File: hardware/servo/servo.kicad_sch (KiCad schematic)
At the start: 51 parts, among them J2 Conn_ARM_SWD_TagConnect_TC203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, U3 DRV8876PWPR, U4 STM32G030F6P6, U5 SIT3088EEUA, U6 SRV05-4

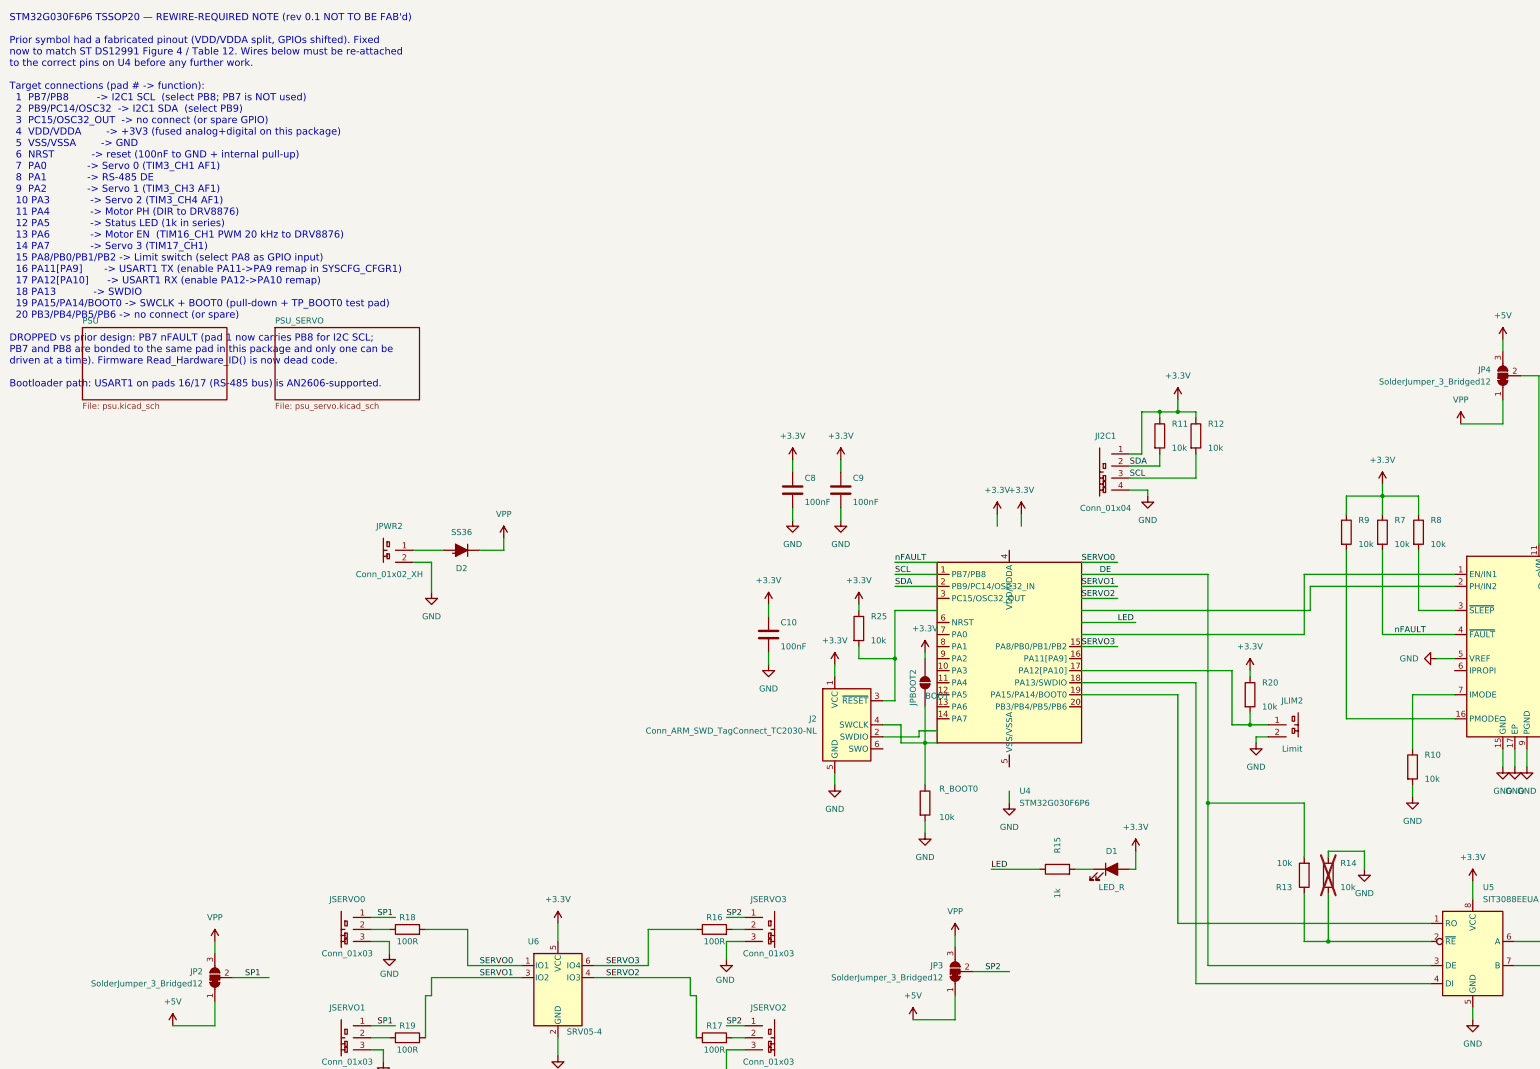
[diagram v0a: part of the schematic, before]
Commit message: hw/servo: regen docs + JLCPCB package after rewire
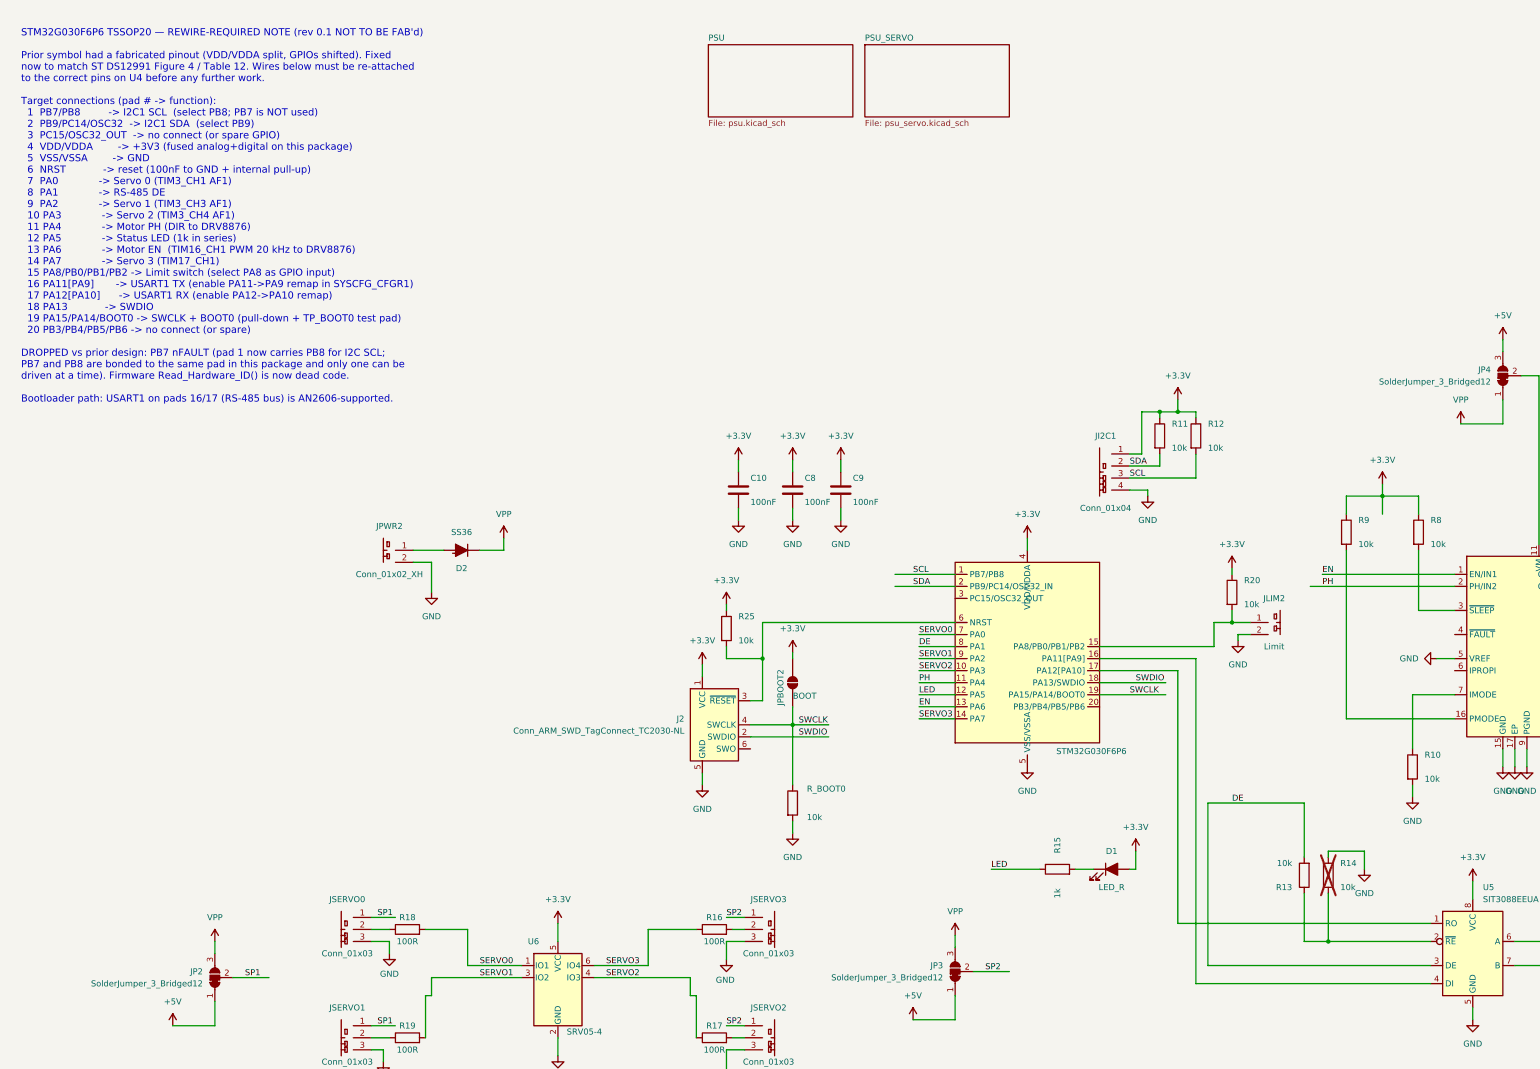
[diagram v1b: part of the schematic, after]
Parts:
- removed R7: 10k, Resistor_SMD:R_0402_1005Metric, symbol Device:R
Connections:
- net +3.3V: now also U4.4 (VDD/VDDA)
- net DE: now also U4.8 (PA1)
- net GND: now also U4.5 (VSS/VSSA)
- net LED: now also U4.12 (PA5)
- net SERVO0: now also U4.7 (PA0)
- net SERVO1: now also U4.9 (PA2)
- net SERVO2: now also U4.10 (PA3)
- net SERVO3: now also U4.14 (PA7); no longer U4.15 (PA8/PB0/PB1/PB2)
- net SWDIO: now reaches J2.2 (SWDIO)
- net SWDIO: now also U4.18 (PA13/SWDIO)
- net at J2.3 (~{RESET}), R25.2: now also U4.6 (NRST)
- net SWCLK: now reaches J2.4 (SWCLK), JPBOOT2.1 (A), R_BOOT0.1
- net SWCLK: now also U4.19 (PA15/PA14/BOOT0)
- net PH: now reaches U4.11 (PA4)
- net PH: now also U3.2 (PH/IN2)
- net EN: now reaches U4.13 (PA6)
- net EN: now also U3.1 (EN/IN1)
- net at U4.16 (PA11[PA9]): now also U5.4 (DI)
- net at JLIM2.1 (Pin_1), R20.2: now also U4.15 (PA8/PB0/PB1/PB2); no longer U4.17 (PA12[PA10])
- net at U5.1 (RO): now also U4.17 (PA12[PA10]); no longer U4.19 (PA15/PA14/BOOT0)
- net nFAULT: no longer names the net of U3.4 (~{FAULT})
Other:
- moved on the sheet: C10, J2, JLIM2, JPBOOT2, R20, R25, R_BOOT0
